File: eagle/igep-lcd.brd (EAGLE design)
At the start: 108.9 x 68.6 mm, 68 parts, among them IC1 LM1117IMPX-3.3, U1 SN74LVC8T245PW, U2 SN74LVC8T245PW, U3 SN74LVC8T245PW, U4 SN74LVC8T245PW

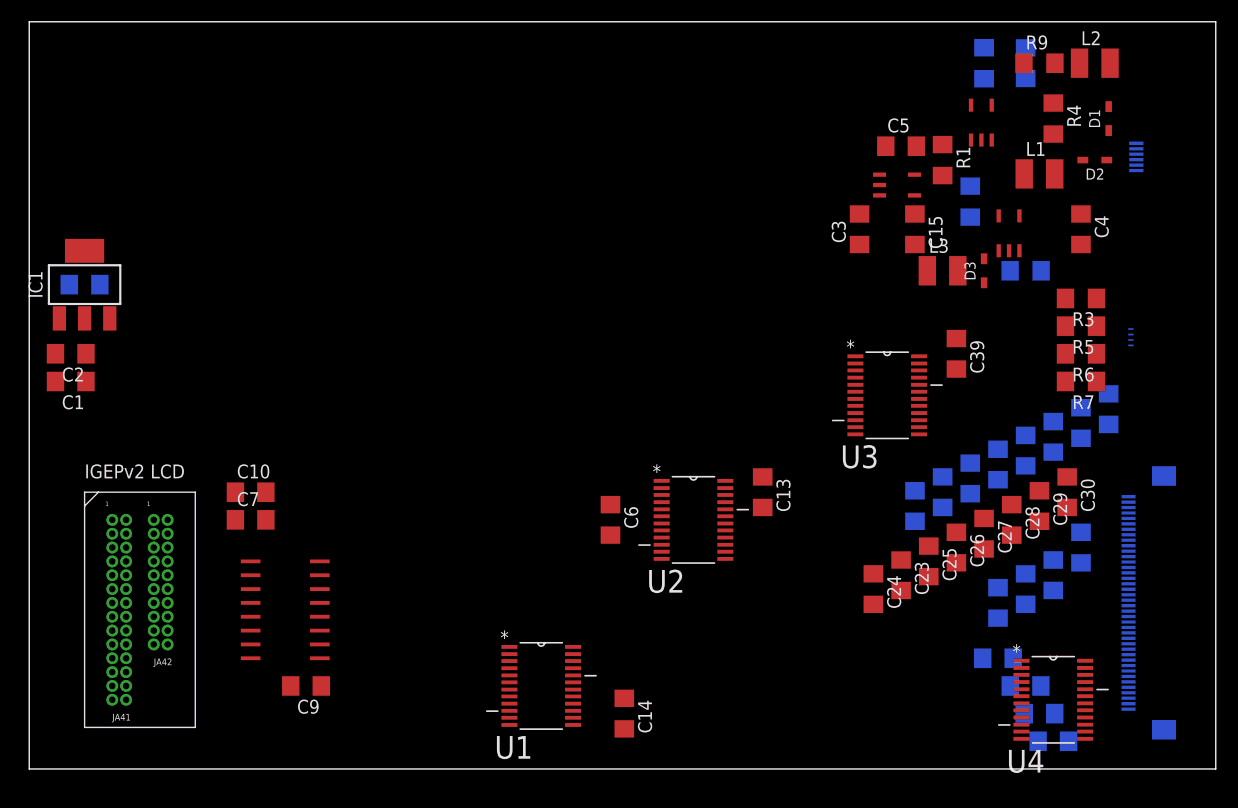
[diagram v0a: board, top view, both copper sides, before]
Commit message: First routed version of the PCB
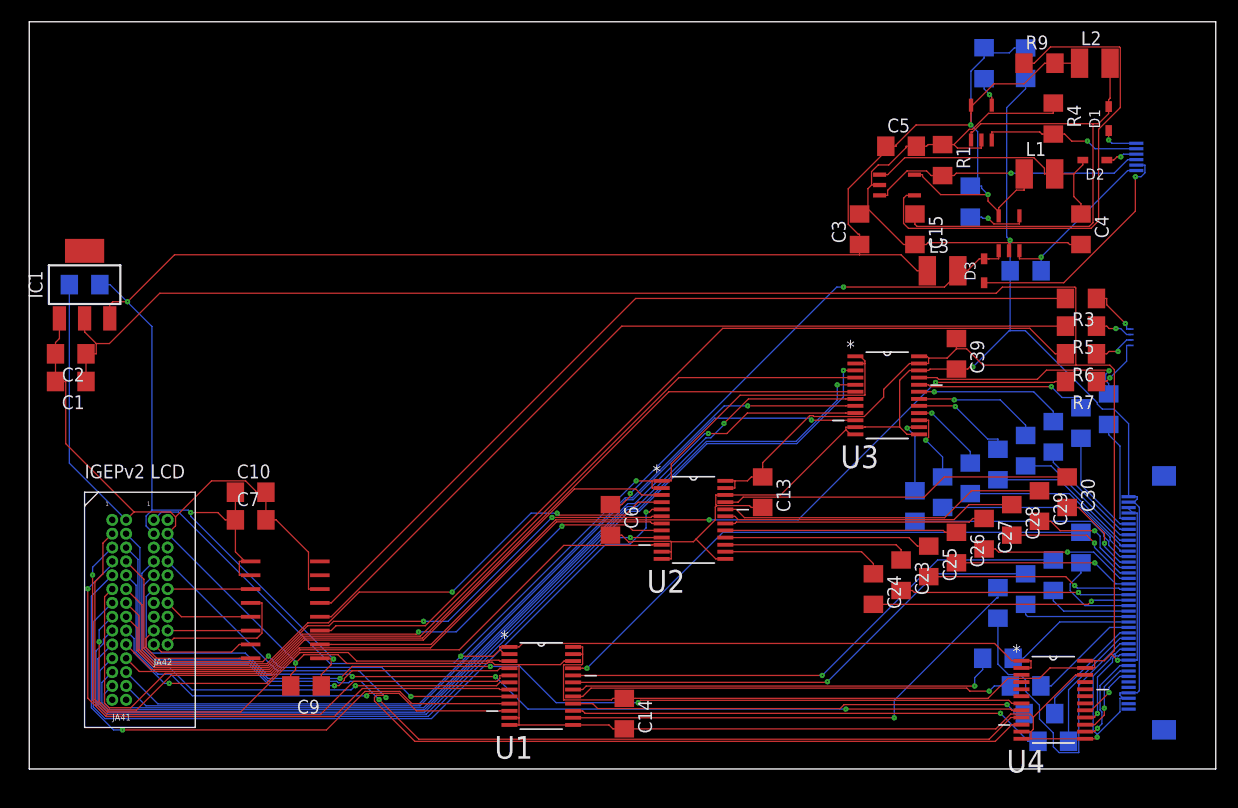
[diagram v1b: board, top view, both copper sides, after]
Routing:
- net N$2: track 0.00 -> 387.7 mm, vias 0 -> 4
- net N$36: track 0.00 -> 258.2 mm, vias 0 -> 1
- net N$35: track 0.00 -> 214.4 mm, vias 0 -> 5
- net N$4: track 0.00 -> 145.2 mm, vias 0 -> 2
- net VSYNC: track 0.00 -> 93.6 mm, vias 0 -> 1
- net DEN: track 0.00 -> 90.8 mm, vias 0 -> 3
- net IGEP_LCD_DATA16: track 0.00 -> 90.5 mm, vias 0 -> 1
- net PCLK: track 0.00 -> 88.4 mm, vias 0 -> 3
- net HSYNC\: track 0.00 -> 88.3 mm, vias 0 -> 1
- net IGEP_LCD_DATA18: track 0.00 -> 87.6 mm, vias 0 -> 1
- net IGEP_LCD_DATA20: track 0.00 -> 84.5 mm, vias 0 -> 1
- net IGEP_LCD_DATA22: track 0.00 -> 82.2 mm, vias 0 -> 1
- net N$33: track 0.00 -> 80.9 mm
- net N$29: track 0.00 -> 80.0 mm
- net N$31: track 0.00 -> 79.5 mm
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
